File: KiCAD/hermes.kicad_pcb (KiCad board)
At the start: 2 copper layers, 32.8 x 53.6 mm, 8 parts, among them U1 MPU-6500, U2 XIAO-RP2040-DIP

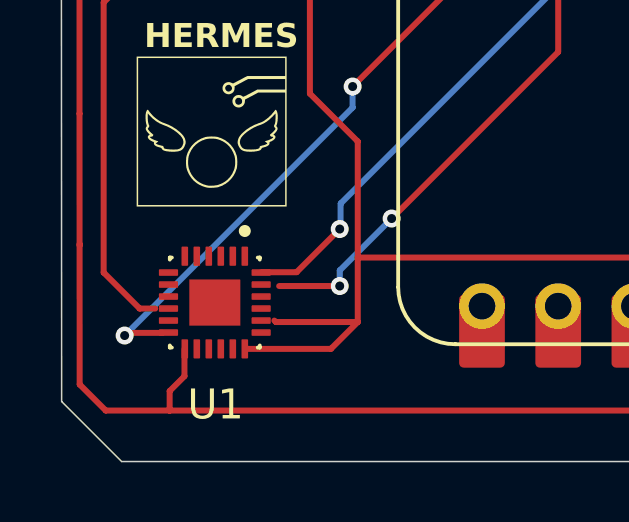
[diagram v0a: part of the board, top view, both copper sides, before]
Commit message: step 3 + 4
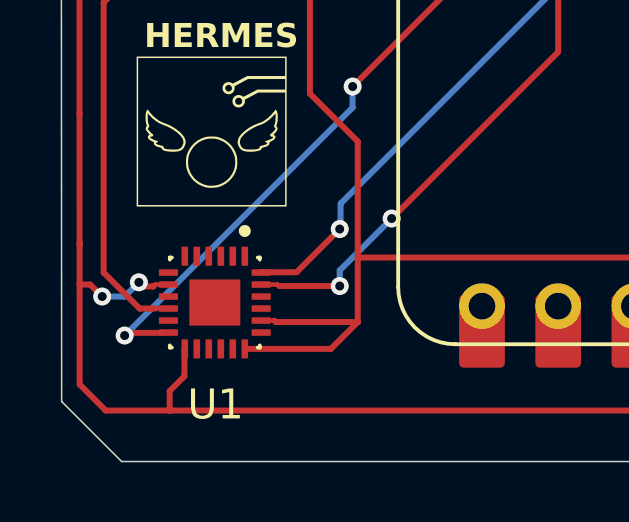
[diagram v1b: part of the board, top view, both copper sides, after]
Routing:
- net 3V3: track 90.2 -> 93.6 mm, vias 0 -> 2
- net SCL: track 49.1 -> 49.7 mm
- net Net-(U1-REGOUT): track 14.6 -> 15.2 mm
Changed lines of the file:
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@@
+	)
+	(segment
+		(start 101.16 122.5)
+		(end 100.6 122.5)
+		(width 0.15)
+		(layer "F.Cu")
+		(net 1)
 	)
 	(segment
@@
 	(segment
 		(start 100.2 122.5)
-		(end 100.719666 122.5)
+		(end 100.6 122.5)
 		(width 0.2)
 		(layer "F.Cu")
@@
 	)
 	(segment
+		(start 100.6 122.5)
+		(end 100.719666 122.5)
+		(width 0.2)
+		(layer "F.Cu")
+		(net 1)
+	)
+	(segment
+		(start 104.25 122.9)
+		(end 104.690334 122.9)
+		(width 0.15)
+		(layer "F.Cu")
+		(net 2)
+	)
+	(segment
 		(start 107.47 122.95)
 		(end 107.47 120.8)
@@
 	(segment
 		(start 98.197855 120.4)
-		(end 98.200656 125.030656)
+		(end 98.198641 121.7)
 		(width 0.2)
 		(layer "F.Cu")
@@
 	)
 	(segment
+		(start 98.198641 121.7)
+		(end 98.200656 125.030656)
+		(width 0.2)
+		(layer "F.Cu")
+		(net 3)
+	)
+	(segment
 		(start 101.005 107.39)
 		(end 99.795 108.6)
@@
 	)
 	(segment
+		(start 98.55147 121.7)
+		(end 98.950735 122.099265)
+		(width 0.2)
+		(layer "F.Cu")
+		(net 3)
+	)
+	(segment
 		(start 100.895 104.56)
 		(end 99 102.665)
@@
 	)
 	(segment
+		(start 100.174265 121.625735)
+		(end 100.313697 121.765167)
+		(width 0.2)
+		(layer "F.Cu")
+		(net 3)
+	)
+	(segment
+		(start 98.198641 121.7)
+		(end 98.55147 121.7)
+		(width 0.2)
+		(layer "F.Cu")
+		(net 3)
+	)
+	(segment
 		(start 99 81.6)
 		(end 103.2 77.4)
@@
 	)
 	(segment
+		(start 101.16 121.7)
+		(end 100.719666 121.7)
+		(width 0.15)
+		(layer "F.Cu")
+		(net 3)
+	)
+	(segment
+		(start 100.313697 121.765167)
+		(end 100.654499 121.765167)
+		(width 0.2)
+		(layer "F.Cu")
+		(net 3)
+	)
+	(segment
 		(start 121.7715 123.255)
 		(end 119.1265 125.9)
@@
 	)
 	(segment
+		(start 100.719666 121.7)
+		(end 100.654499 121.765167)
+		(width 0.15)
+		(layer "F.Cu")
+		(net 3)
+	)
+	(segment
+		(start 100.654499 121.765167)
+		(end 100.659833 121.759833)
+		(width 0.2)
+		(layer "F.Cu")
+		(net 3)
+	)
+	(segment
 		(start 99 108.6)
 		(end 99 110.8)
@@
 		(width 0.2)
 		(layer "F.Cu")
+		(net 3)
+	)
+	(via
+		(at 98.950735 122.099265)
+		(size 0.6)
+		(drill 0.3)
+		(layers "F.Cu" "B.Cu")
+		(net 3)
+	)
+	(via
+		(at 100.174265 121.625735)
+		(size 0.6)
+		(drill 0.3)
+		(layers "F.Cu" "B.Cu")
+		(net 3)
+	)
+	(segment
+		(start 98.950735 122.099265)
+		(end 99.700735 122.099265)
+		(width 0.2)
+		(layer "B.Cu")
+		(net 3)
+	)
+	(segment
+		(start 99.700735 122.099265)
+		(end 100.174265 121.625735)
+		(width 0.2)
+		(layer "B.Cu")
 		(net 3)
 	)
@@
 	)
 	(segment
+		(start 104.8 121.7)
+		(end 104.85 121.75)
+		(width 0.15)
+		(layer "F.Cu")
+		(net 5)
+	)
+	(segment
 		(start 106.87 121.75)
 		(end 104.85 121.75)
@@
 		(layer "F.Cu")
 		(net 5)
+	)
+	(segment
+		(start 104.25 121.7)
+		(end 104.8 121.7)
+		(width 0.15)
+		(layer "F.Cu")
+		(net 5)
